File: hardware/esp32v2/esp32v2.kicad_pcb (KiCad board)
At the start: 2 copper layers, 21 x 29.8 mm, 32 parts, among them J2 Conn_01x02, J3 Conn_01x10, U1 ESP32-S3, U3 W25Q128JVS, Y1 32.768 kHz, Y2 40MHz(10ppm)

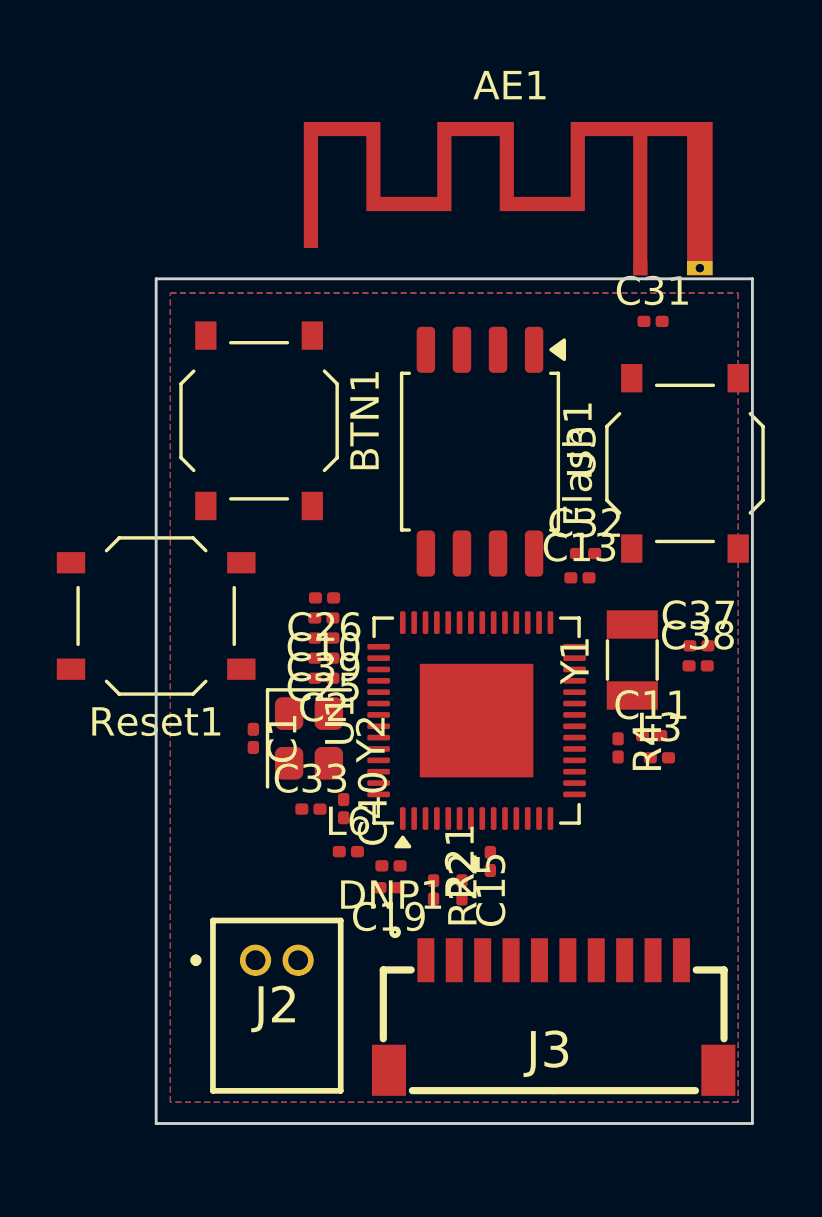
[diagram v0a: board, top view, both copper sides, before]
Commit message: wip
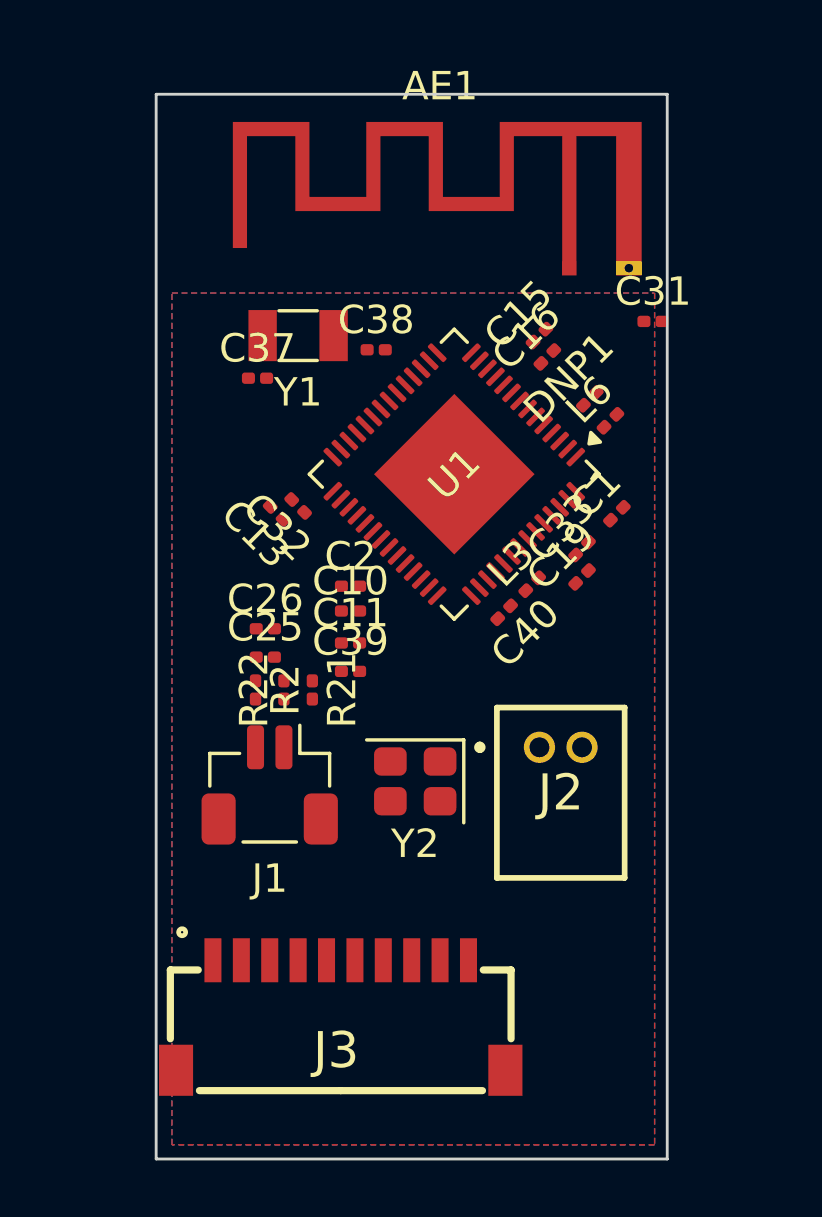
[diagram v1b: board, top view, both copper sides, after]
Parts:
- removed BTN1: BTN, Button_Switch_SMD:SW_Push_1P1T_XKB_TS-1187A
- removed Flash1: Flash, Button_Switch_SMD:SW_Push_1P1T_XKB_TS-1187A
- removed R4: 10K, Resistor_SMD:R_0201_0603Metric
- removed Reset1: Reset, Button_Switch_SMD:SW_Push_1P1T_XKB_TS-1187A
- removed U3: W25Q128JVS, Package_SO:SOIC-8_5.3x5.3mm_P1.27mm
- added C16: 0.1uF, Capacitor_SMD:C_0201_0603Metric, F.Cu at (115.8, 35.3)
- added J1: Conn_01x02, Connector_JST:JST_SH_BM02B-SRSS-TB_1x02-1MP_P1.00mm_Vertical, F.Cu at (106.0, 50.3)
- added R2: 10K, Resistor_SMD:R_0201_0603Metric, F.Cu at (105.5, 47.0)
- moved C15 19.7 mm to (115.5, 34.5), turned to 45 degrees
- moved C37 18.2 mm to (105.6, 36.0)
- moved DNP1 17.9 mm to (117.3, 36.7), turned to 45 degrees
- moved L6 17.8 mm to (118.0, 37.5), turned to 45 degrees
- moved Y1 16.4 mm to (107.0, 34.5), turned to 180 degrees
- moved C38 15.9 mm to (109.8, 35.0)
- moved C1 15.1 mm to (118.2, 40.8), turned to 45 degrees
- moved C33 13.2 mm to (117.0, 42.0), turned to 45 degrees
- moved C19 12.9 mm to (117.0, 43.0), turned to 45 degrees
- moved J2 12.5 mm to (115.5, 49.0)
- moved C11 11.1 mm to (108.8, 45.3)
- moved C13 10.9 mm to (106.2, 40.7), turned to 135 degrees
- moved C32 10.3 mm to (107.0, 40.5), turned to 135 degrees
- moved C40 8.93 mm to (114.3, 44.2), turned to -135 degrees
- moved R22 8.79 mm to (106.5, 47.0), turned to 90 degrees
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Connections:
- J2 pad 1: GND -> VDD_CPU
- J2 pad 2: VDD_CPU -> GND
- J3 pad 1: IO1 -> USB_D-
- J3 pad 10: USB_D+ -> IO1
- J3 pad 2: IO2 -> USB_D+
- J3 pad 3: IO3 -> IO8
- J3 pad 4: IO4/BAT -> IO7
- J3 pad 5: IO5 -> IO6
- J3 pad 6: IO6 -> IO5
- J3 pad 7: IO7 -> IO4/BAT
- J3 pad 8: IO8 -> IO3
- J3 pad 9: USB_D- -> IO2
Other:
- board size 21 x 29.8 mm -> 18 x 37.5 mm

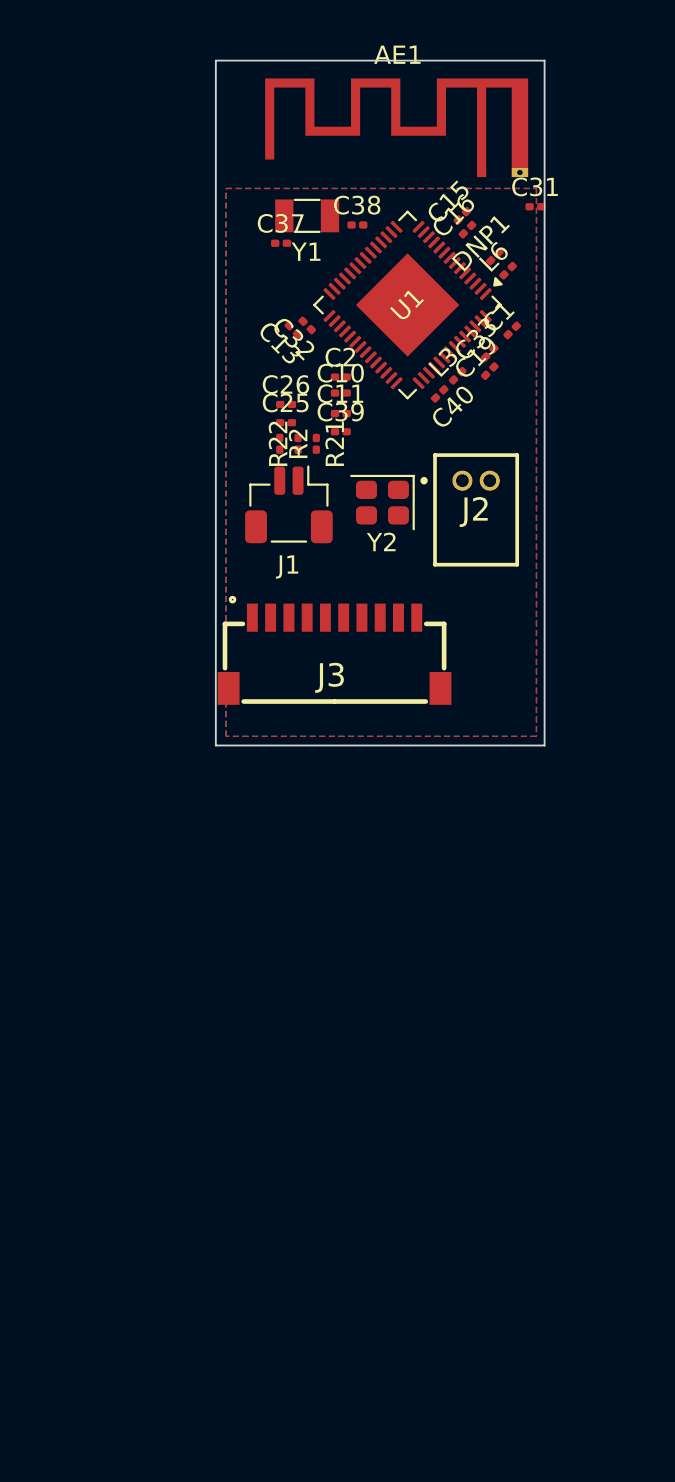
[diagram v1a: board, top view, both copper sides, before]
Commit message: wip
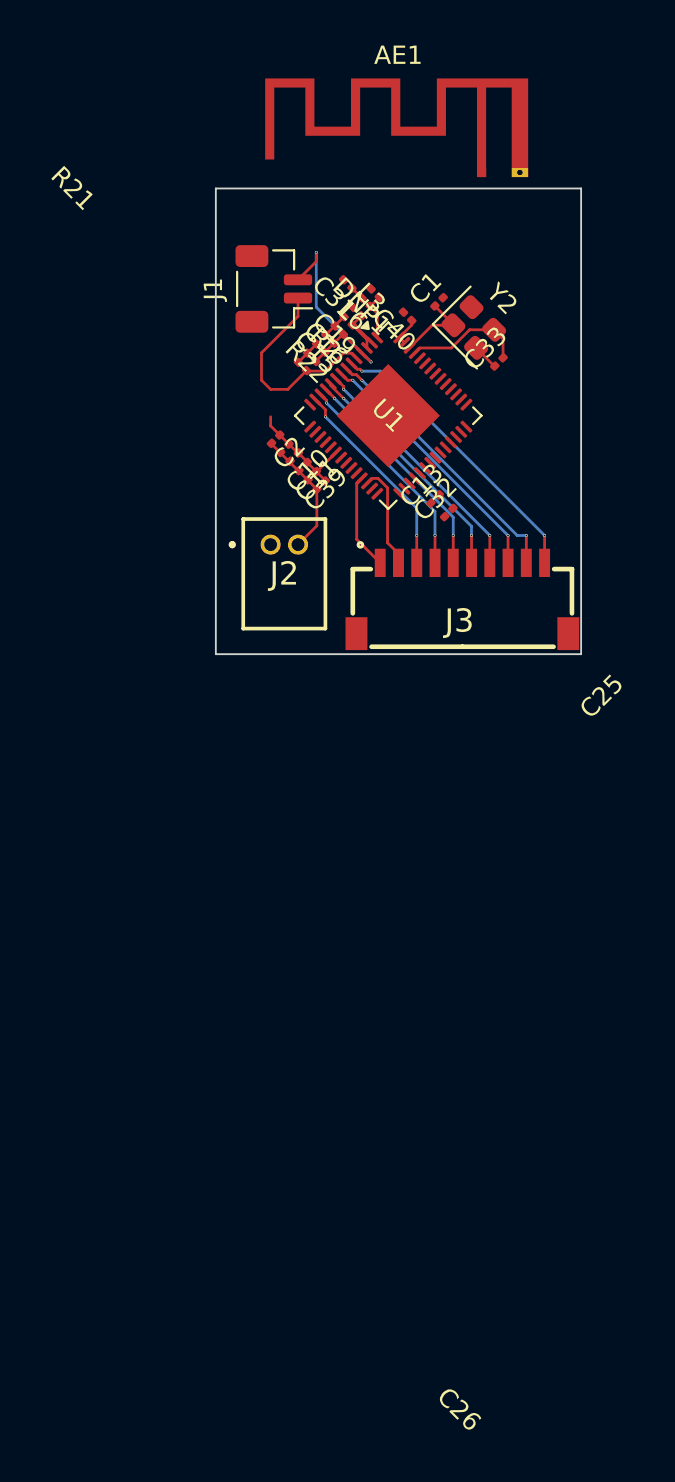
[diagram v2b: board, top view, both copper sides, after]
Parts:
- removed C37, C38: 12pF, Capacitor_SMD:C_0201_0603Metric
- removed Y1: 32.768 kHz, Crystal:Crystal_SMD_3215-2Pin_3.2x1.5mm
- moved C32 12.8 mm to (114.8, 50.7), turned to 45 degrees
- moved C13 12.1 mm to (114.0, 50.0), turned to 45 degrees
- moved J1 11.9 mm to (105.2, 38.5), turned to 90 degrees
- moved C31 11.1 mm to (109.2, 38.2), turned to 135 degrees
- moved J2 11.1 mm to (105.0, 52.5)
- moved Y2 10.8 mm to (116.1, 40.6), turned to -45 degrees
- moved C15 9.91 mm to (108.2, 41.2), turned to 135 degrees
- moved C16 8.92 mm to (108.8, 40.8), turned to 135 degrees
- moved C19 8.23 mm to (109.2, 40.2), turned to 135 degrees
- moved L6 7.96 mm to (110.2, 39.2), turned to 135 degrees
- moved J3 7.62 mm to (109.5, 53.8)
- moved DNP1 6.85 mm to (110.7, 38.7), turned to 135 degrees
- moved L3 6.53 mm to (109.7, 39.7), turned to -45 degrees
- moved U1 6.15 mm to (111.4, 45.4), turned to -45 degrees
- moved R22 5.38 mm to (107.7, 41.7), turned to 135 degrees
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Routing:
- net IO1: track 0.00 -> 16.0 mm, vias 0 -> 2
- net IO2: track 0.00 -> 15.1 mm, vias 0 -> 2
- net IO3: track 0.00 -> 14.3 mm, vias 0 -> 2
- net IO4/BAT: track 0.00 -> 13.6 mm, vias 0 -> 2
- net EN: track 0.00 -> 13.4 mm, vias 0 -> 2
- net IO5: track 0.00 -> 13.0 mm, vias 0 -> 2
- net IO6: track 0.00 -> 12.4 mm, vias 0 -> 2
- net IO7: track 0.00 -> 11.8 mm, vias 0 -> 2
- net IO0: track 0.00 -> 11.7 mm
- net IO8: track 0.00 -> 11.2 mm, vias 0 -> 2
- net GND: track 0.00 -> 9.86 mm
- net VDD_CPU: track 0.00 -> 9.32 mm
- net Net-(U1-XTAL_N): track 0.00 -> 6.69 mm
- net USB_D+: track 0.00 -> 5.81 mm
- net USB_D-: track 0.00 -> 5.28 mm
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- removed copper zone on B.Cu, net GND
- removed copper zone on F.Cu, net GND
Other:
- board size 18 x 37.5 mm -> 20 x 25.5 mm
- copper layers 2 -> 4
